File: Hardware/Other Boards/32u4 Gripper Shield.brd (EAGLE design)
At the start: 29.2 x 41.9 mm, 22 parts, among them Q1 MOSFET-NCHANNELBSS138, Q2 MOSFET-NCHANNELBSS138, U1 SN74LS241DW, U2 XBEE-1B3, U3 V_REG_LDOSMD

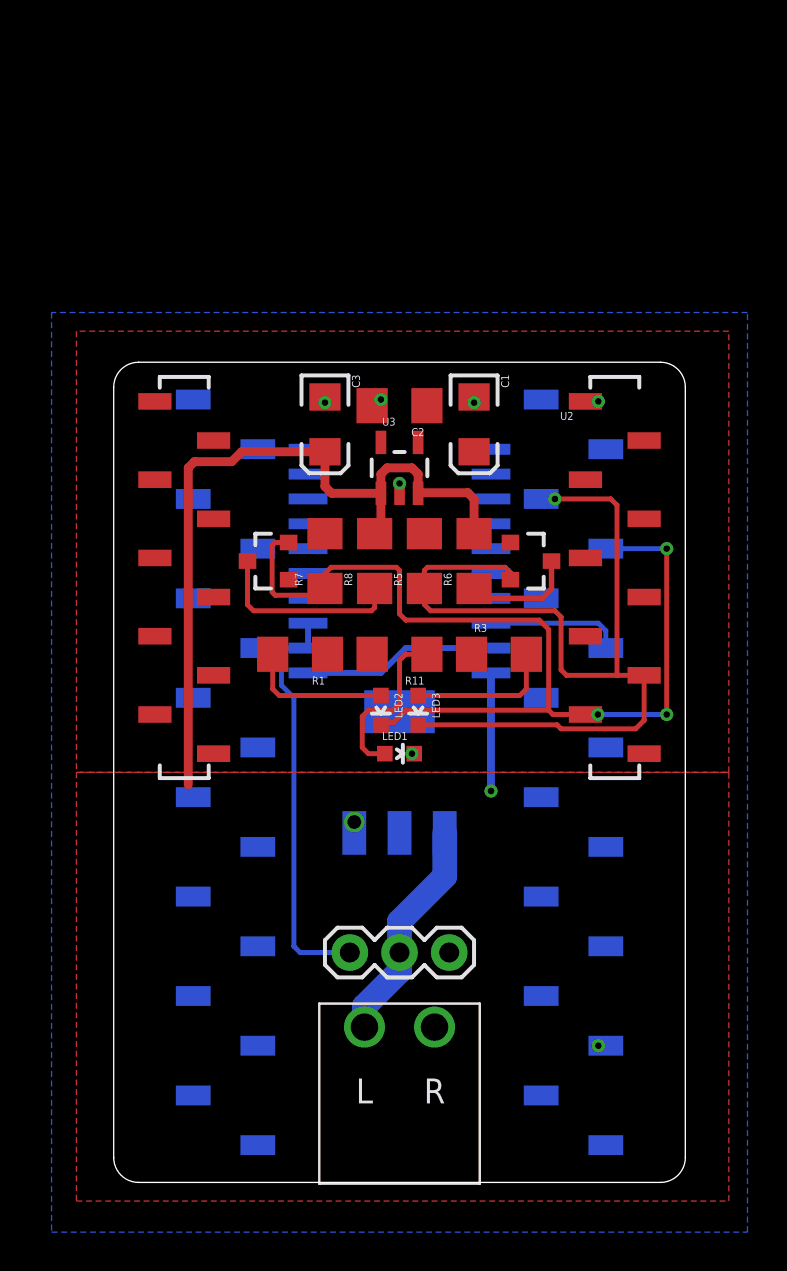
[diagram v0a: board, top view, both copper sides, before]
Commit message: Finished gripper shield
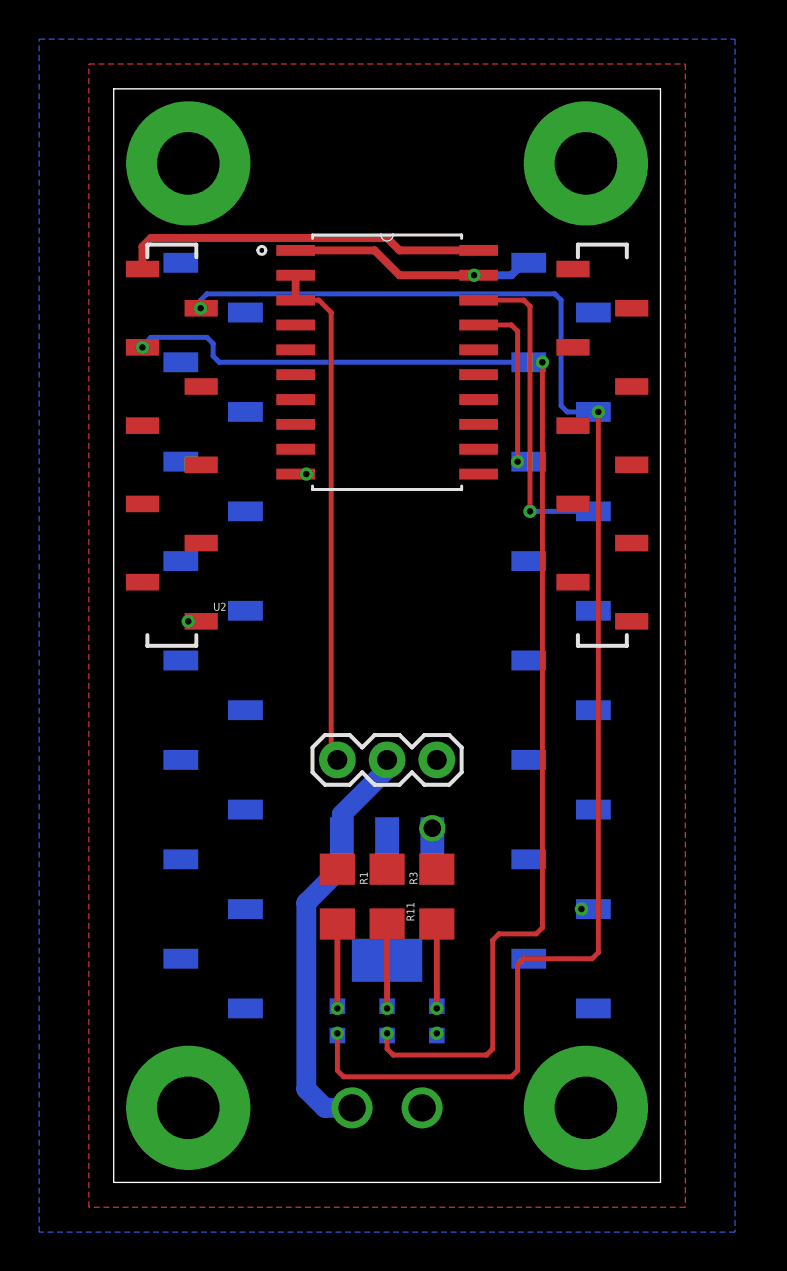
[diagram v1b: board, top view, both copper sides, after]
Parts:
- removed C1, C3: 10uF, SparkFun:EIA3216
- removed C2: 0.1uF, SparkFun-Passives:1206
- removed Q1, Q2: MOSFET-NCHANNELBSS138, SparkFun-DiscreteSemi:SOT23-3
- removed R5, R6, R7, R8: 1k, SparkFun-Passives:1206
- removed U3: V_REG_LDOSMD, SparkFun:SOT23-5
- added S1, S2, S3, S4: STANDOFF_ELECTRICAL, SparkFun-Electromechanical:STANDOFF-ELECTRICAL
- U$3: value H_WR-TBL_321*0002HORIZ -> H_WR-TBL_321*0002VERT; device MRDT-2015-PowerBoard:691322110002 -> MRDT-2015-PowerBoard:691321100002
- moved LED2 16.0 mm to (11.4, 8.26), flipped to the bottom
- moved LED3 16.0 mm to (14.0, 8.26), flipped to the bottom
- moved U2 15.3 mm to (14.0, 26.7), turned to 0 degrees
- moved LED1 13.8 mm to (16.5, 8.26), flipped to the bottom, turned to 180 degrees
- moved R3 13.6 mm to (14.0, 14.6), turned to 270 degrees
- moved R11 12.5 mm to (16.5, 14.6), turned to 90 degrees
- moved R1 12.5 mm to (11.4, 14.6), turned to 270 degrees
- moved U1 10.2 mm to (14.0, 41.9), flipped to the top, turned to 0 degrees
- moved JP1 9.86 mm to (11.4, 21.6)
- moved U$1 7.01 mm to (14.0, 27.9)
- moved U$5 6.54 mm to (14.0, 14.4), turned to 180 degrees
- moved U$3 4.18 mm to (14.0, 3.81), flipped to the bottom, turned to 180 degrees
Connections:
- removed net 5V: C3.A, R6.2, R8.2, U$1.P$3, U$5.3, U1.20, U3.1, U3.3
- removed net DIN: Q1.3, R6.1
- removed net DOUT: Q2.3, R8.1
- net 3.3V: now also U$1.P$3, U$5.3, U1.20; no longer C1.A, C2.1, Q1.1, Q2.1, R5.2, R7.2, U3.5
- net DC_1: now also U$1.P$16
- net GND: now also S1.P1, S2.P1, S3.P1, S4.P1; no longer C1.C, C2.2, C3.C, U3.2
- net RX_0: no longer Q2.2, R7.1
- net TX_0: no longer Q1.2, R5.1
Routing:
- net 5V: track 46.6 -> 0.00 mm, vias 3 -> 0
- net RX_0: track 52.6 -> 75.5 mm
- net 3.3V: track 0.00 -> 19.9 mm, vias 0 -> 2
- net TX_0: track 47.8 -> 65.9 mm, vias 1 -> 3
- net DOUT: track 9.91 -> 0.00 mm
- net 12V: track 11.6 -> 21.3 mm
- net RX_1: track 6.91 -> 16.5 mm, vias 0 -> 1
- net TX_1: track 2.57 -> 9.36 mm, vias 0 -> 1
- net DIN: track 5.80 -> 0.00 mm
- net DDATA_1: track 20.9 -> 26.3 mm
- net N$38: track 8.80 -> 4.43 mm, vias 0 -> 1
- net DC_1: track 9.87 -> 12.9 mm, vias 0 -> 1
- net N$4: track 7.44 -> 4.43 mm, vias 0 -> 1
- net N$1: track 7.44 -> 4.43 mm, vias 0 -> 1
- net GND: track 2.41 -> 1.32 mm, vias 6 -> 3
- removed copper zone on layer 1, net 5V
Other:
- board size 29.2 x 41.9 mm -> 27.9 x 55.9 mm
